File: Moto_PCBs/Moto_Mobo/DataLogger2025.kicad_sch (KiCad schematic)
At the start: 73 parts, among them J1 2171790001, J2 2908-05WB-MG, J3 0436500201 1x02, J5 0436500201 1x02, J6 0436500201 1x02, J7 B10B-XH-A, SW1 SMD_4.6x2.8mm_h1.9mm, U1 USBLC6-2SC6, U2 SM24CANB-02HTG, U3 SN65HVD230, U4 ESP32-S3-WROOM-1U-N16R8

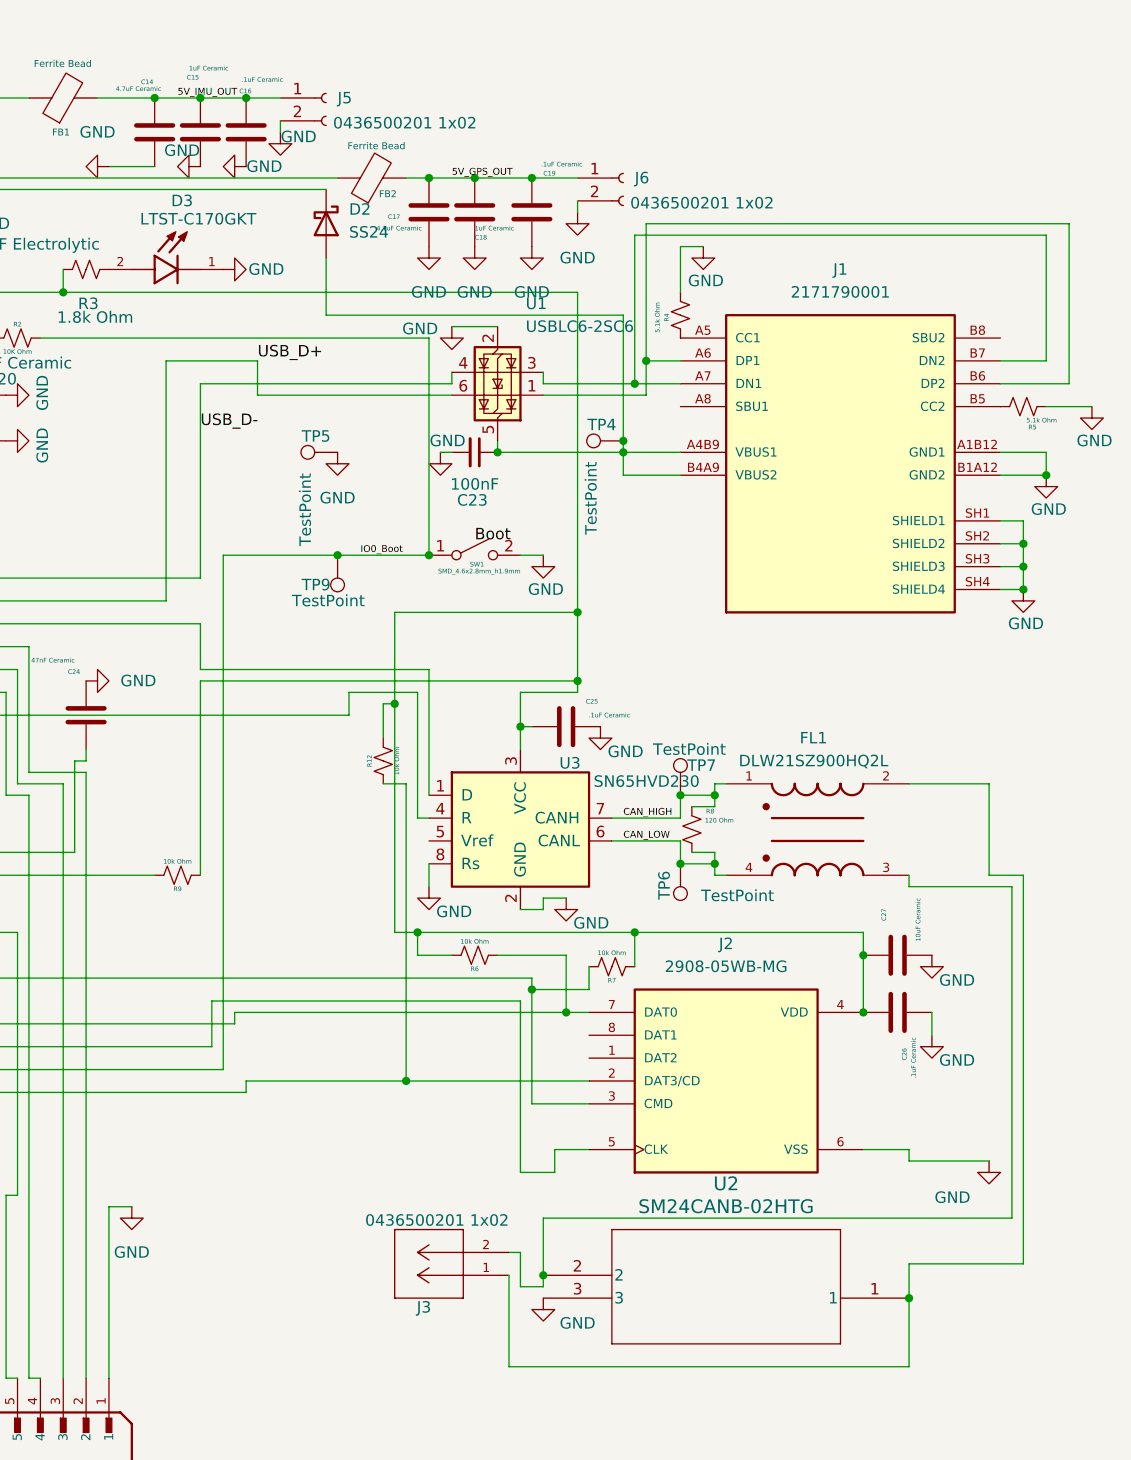
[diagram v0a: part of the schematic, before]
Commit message: Final Mobo GBR/PCB Files before PCBWAY Order
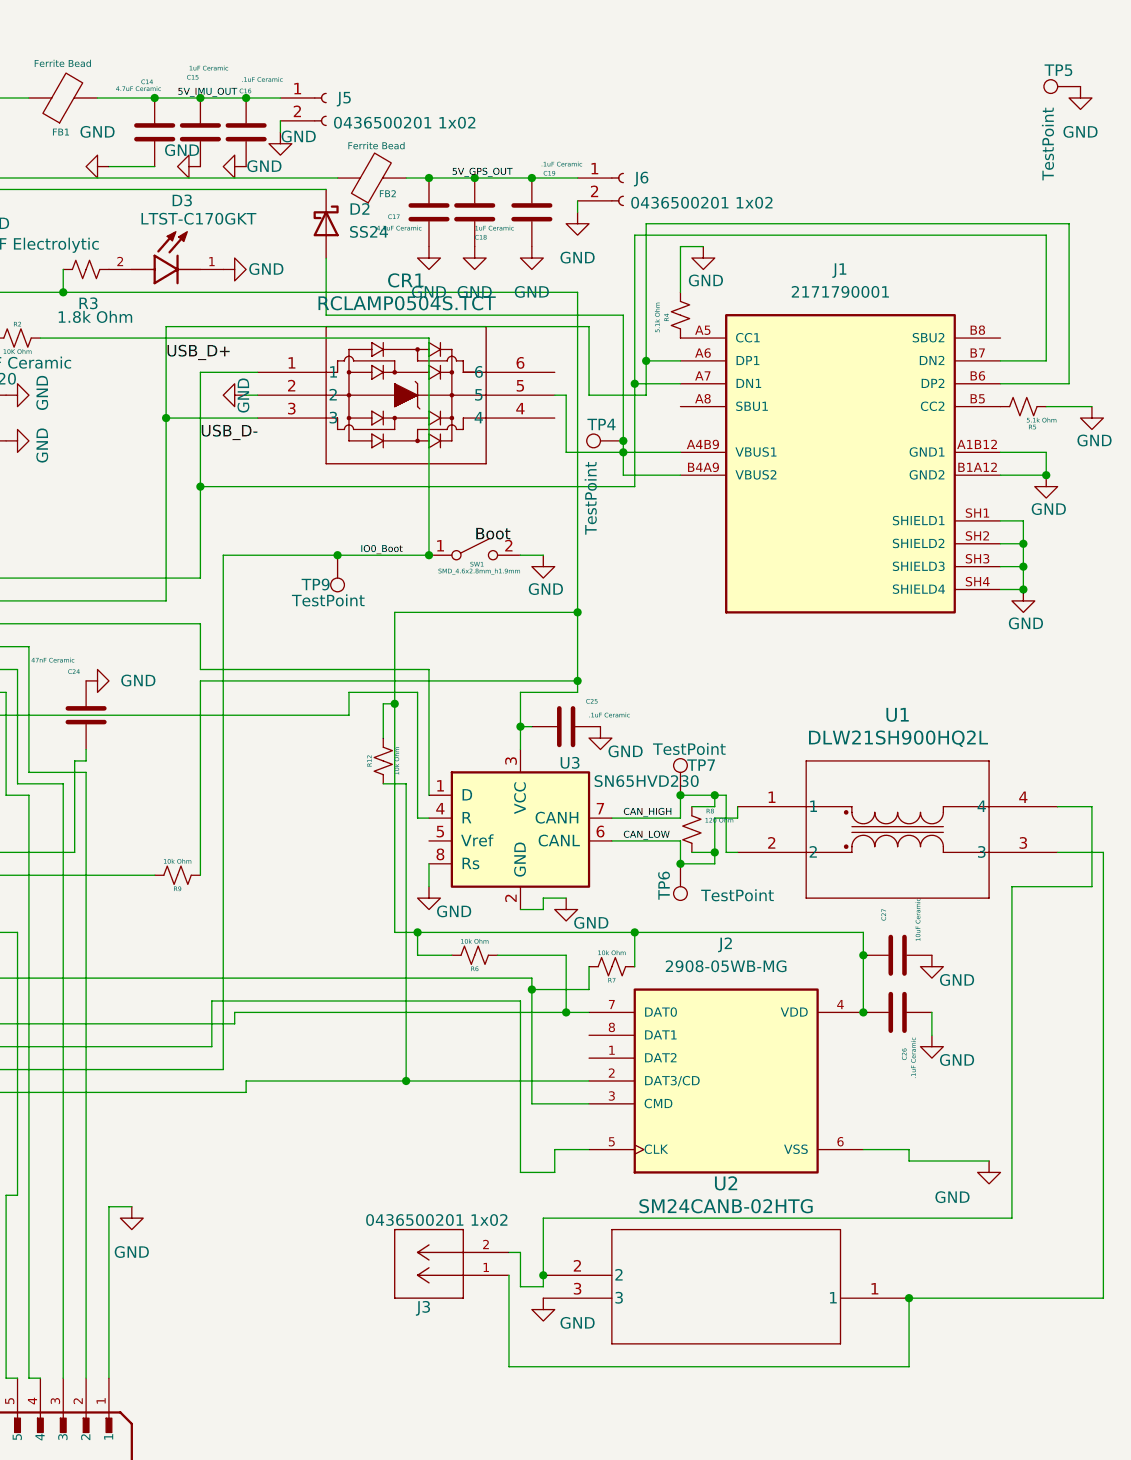
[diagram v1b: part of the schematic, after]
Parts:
- removed C23: 100nF, Capacitor_SMD:C_1206_3216Metric_Pad1.33x1.80mm_HandSolder, symbol Device:C_Small
- removed FL1: DLW21SZ900HQ2L, DLW21SZ900HQ2L:FIL_DLW21SZ900HQ2L, symbol DLW21SZ900HQ2L:DLW21SZ900HQ2L
- removed U1: USBLC6-2SC6, USBLC6-2SC6:SOT95P280X145-6N, symbol Power_Protection:USBLC6-2SC6
- added CR1: RCLAMP0504S.TCT, SC70-6L_RCLAMP_1p75x3p1-0p95_SEM, symbol 2026-06-30_13-10-54:RCLAMP0504S.TCT
- added U1: DLW21SH900HQ2L, DLW21SH900HQ2L:DLW21SH_MUR, symbol 2026-06-30_13-58-37:DLW21SH900HQ2L
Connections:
- net CAN_HIGH: now also U1.2
- net CAN_LOW: now also U1.1
- net GND: now also CR1.2
- net USB_D+: now also J1.A6 (DP1), J1.B6 (DP2), CR1.3
- net USB_D-: now also J1.A7 (DN1), J1.B7 (DN2), CR1.1
- net at J3.1, U2.1: now also U1.3
- net at J3.2, U2.2: now also U1.4
- net at D2.2 (A), J1.A4B9 (VBUS1), J1.B4A9 (VBUS2)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: now also CR1.5
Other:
- moved on the sheet: TP5
